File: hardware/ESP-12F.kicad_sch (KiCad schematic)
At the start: 30 parts, among them J10 PROG_PORT, U10 ESP-12F, U11 MCP2558FD-xMF, U8 PI4IOE5V6416LEX, U9 PI4IOE5V6416LEX

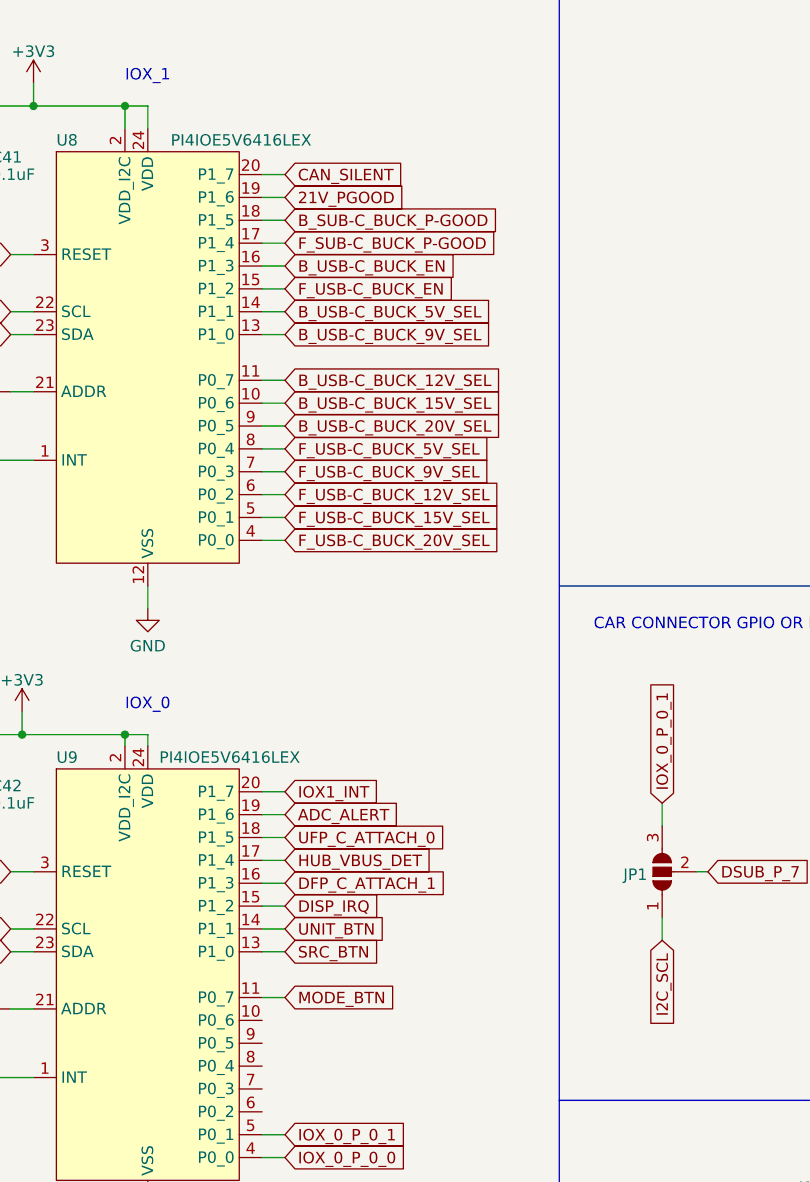
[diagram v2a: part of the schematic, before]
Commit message: coldent sleep so came back and did somre routing
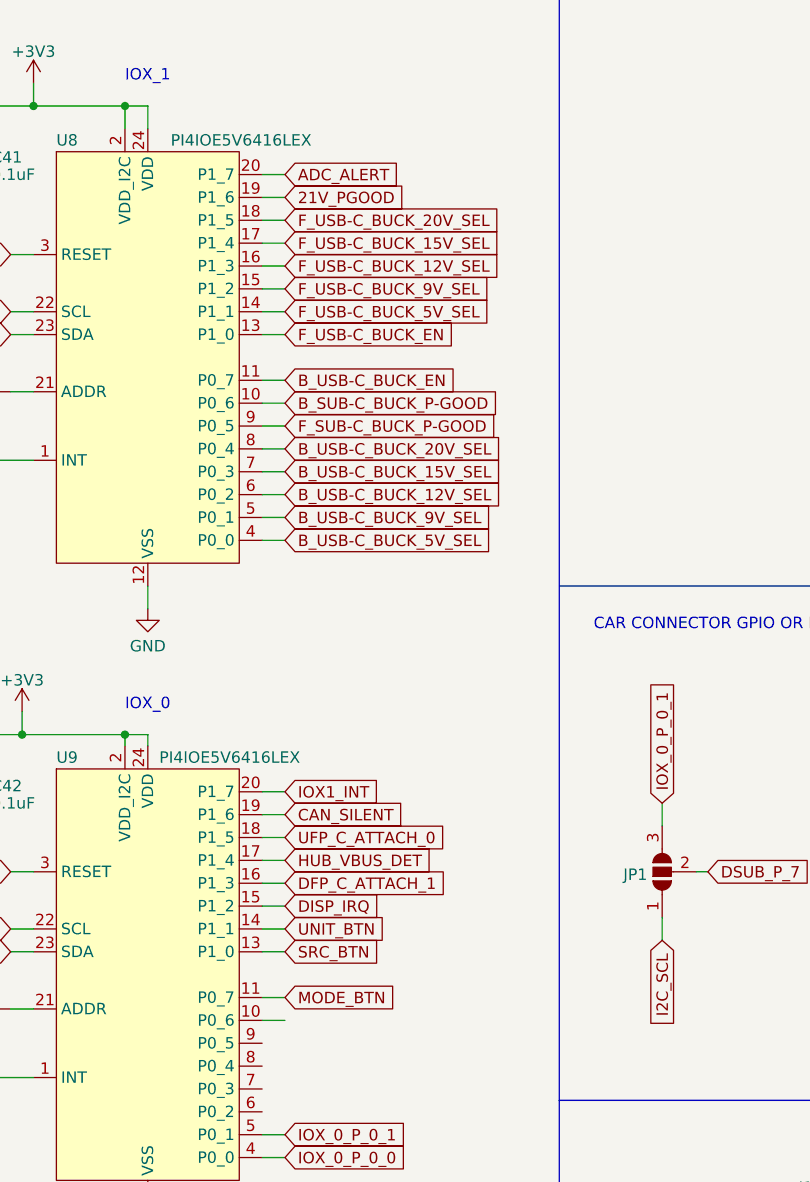
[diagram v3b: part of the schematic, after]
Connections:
- net ADC_ALERT: now also U8.20 (P1_7); no longer U9.19 (P1_6)
- net B_SUB-C_BUCK_P-GOOD: now also U8.10 (P0_6); no longer U8.18 (P1_5)
- net B_USB-C_BUCK_12V_SEL: now also U8.6 (P0_2); no longer U8.11 (P0_7)
- net B_USB-C_BUCK_15V_SEL: now also U8.7 (P0_3); no longer U8.10 (P0_6)
- net B_USB-C_BUCK_20V_SEL: now also U8.8 (P0_4); no longer U8.9 (P0_5)
- net B_USB-C_BUCK_5V_SEL: now also U8.4 (P0_0); no longer U8.14 (P1_1)
- net B_USB-C_BUCK_9V_SEL: now also U8.5 (P0_1); no longer U8.13 (P1_0)
- net B_USB-C_BUCK_EN: now also U8.11 (P0_7); no longer U8.16 (P1_3)
- net CAN_SILENT: now also U9.19 (P1_6); no longer U8.20 (P1_7)
- net F_SUB-C_BUCK_P-GOOD: now also U8.9 (P0_5); no longer U8.17 (P1_4)
- net F_USB-C_BUCK_12V_SEL: now also U8.16 (P1_3); no longer U8.6 (P0_2)
- net F_USB-C_BUCK_15V_SEL: now also U8.17 (P1_4); no longer U8.5 (P0_1)
- net F_USB-C_BUCK_20V_SEL: now also U8.18 (P1_5); no longer U8.4 (P0_0)
- net F_USB-C_BUCK_5V_SEL: now also U8.14 (P1_1); no longer U8.8 (P0_4)
- net F_USB-C_BUCK_9V_SEL: now also U8.15 (P1_2); no longer U8.7 (P0_3)
- net F_USB-C_BUCK_EN: now also U8.13 (P1_0); no longer U8.15 (P1_2)
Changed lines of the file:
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@@
+    (stroke (width 0) (type default))
+  )
+  (wire (pts (xy 82.55 50.8) (xy 85.09 50.8))
     (stroke (width 0) (type default))
   )
@@
     (stroke (width 0) (type default))
   )
+  (wire (pts (xy 82.55 144.78) (xy 85.09 144.78))
+    (stroke (width 0) (type default))
+  )
   (wire (pts (xy 243.84 33.02) (xy 243.84 35.56))
     (stroke (width 0) (type default))
@@
   )
   (wire (pts (xy 38.1 148.59) (xy 38.1 151.13))
-    (stroke (width 0) (type default))
-  )
-  (wire (pts (xy 82.55 50.8) (xy 85.09 50.8))
     (stroke (width 0) (type default))
   )
@@
     )
   )
-  (global_label "B_SUB-C_BUCK_P-GOOD" (shape input) (at 85.09 55.88 0) (fields_autoplaced)
-    (effects (font (size 1.27 1.27)) (justify left))
-    (property "Intersheetrefs" "${INTERSHEET_REFS}" (at 112.0049 55.88 0)
+  (global_label "B_SUB-C_BUCK_P-GOOD" (shape input) (at 85.09 76.2 0) (fields_autoplaced)
+    (effects (font (size 1.27 1.27)) (justify left))
+    (property "Intersheetrefs" "${INTERSHEET_REFS}" (at 112.0049 76.2 0)
       (effects (font (size 1.27 1.27)) (justify left) hide)
     )
@@
     )
   )
-  (global_label "F_USB-C_BUCK_EN" (shape input) (at 85.09 63.5 0) (fields_autoplaced)
-    (effects (font (size 1.27 1.27)) (justify left))
-    (property "Intersheetrefs" "${INTERSHEET_REFS}" (at 106.2596 63.5 0)
-      (effects (font (size 1.27 1.27)) (justify left) hide)
-    )
-  )
-  (global_label "F_USB-C_BUCK_12V_SEL" (shape input) (at 85.09 86.36 0) (fields_autoplaced)
-    (effects (font (size 1.27 1.27)) (justify left))
-    (property "Intersheetrefs" "${INTERSHEET_REFS}" (at 111.6419 86.36 0)
-      (effects (font (size 1.27 1.27)) (justify left) hide)
-    )
-  )
-  (global_label "B_USB-C_BUCK_15V_SEL" (shape input) (at 85.09 76.2 0) (fields_autoplaced)
-    (effects (font (size 1.27 1.27)) (justify left))
-    (property "Intersheetrefs" "${INTERSHEET_REFS}" (at 111.8233 76.2 0)
-      (effects (font (size 1.27 1.27)) (justify left) hide)
-    )
-  )
-  (global_label "F_USB-C_BUCK_5V_SEL" (shape input) (at 85.09 81.28 0) (fields_autoplaced)
-    (effects (font (size 1.27 1.27)) (justify left))
-    (property "Intersheetrefs" "${INTERSHEET_REFS}" (at 110.4324 81.28 0)
+  (global_label "F_USB-C_BUCK_EN" (shape input) (at 85.09 68.58 0) (fields_autoplaced)
+    (effects (font (size 1.27 1.27)) (justify left))
+    (property "Intersheetrefs" "${INTERSHEET_REFS}" (at 106.2596 68.58 0)
+      (effects (font (size 1.27 1.27)) (justify left) hide)
+    )
+  )
+  (global_label "F_USB-C_BUCK_12V_SEL" (shape input) (at 85.09 60.96 0) (fields_autoplaced)
+    (effects (font (size 1.27 1.27)) (justify left))
+    (property "Intersheetrefs" "${INTERSHEET_REFS}" (at 111.6419 60.96 0)
+      (effects (font (size 1.27 1.27)) (justify left) hide)
+    )
+  )
+  (global_label "B_USB-C_BUCK_15V_SEL" (shape input) (at 85.09 83.82 0) (fields_autoplaced)
+    (effects (font (size 1.27 1.27)) (justify left))
+    (property "Intersheetrefs" "${INTERSHEET_REFS}" (at 111.8233 83.82 0)
+      (effects (font (size 1.27 1.27)) (justify left) hide)
+    )
+  )
+  (global_label "F_USB-C_BUCK_5V_SEL" (shape input) (at 85.09 66.04 0) (fields_autoplaced)
+    (effects (font (size 1.27 1.27)) (justify left))
+    (property "Intersheetrefs" "${INTERSHEET_REFS}" (at 110.4324 66.04 0)
       (effects (font (size 1.27 1.27)) (justify left) hide)
     )
@@
     )
   )
-  (global_label "B_USB-C_BUCK_5V_SEL" (shape input) (at 85.09 66.04 0) (fields_autoplaced)
-    (effects (font (size 1.27 1.27)) (justify left))
-    (property "Intersheetrefs" "${INTERSHEET_REFS}" (at 110.6138 66.04 0)
+  (global_label "B_USB-C_BUCK_5V_SEL" (shape input) (at 85.09 91.44 0) (fields_autoplaced)
+    (effects (font (size 1.27 1.27)) (justify left))
+    (property "Intersheetrefs" "${INTERSHEET_REFS}" (at 110.6138 91.44 0)
       (effects (font (size 1.27 1.27)) (justify left) hide)
     )
@@
     )
   )
-  (global_label "F_USB-C_BUCK_9V_SEL" (shape input) (at 85.09 83.82 0) (fields_autoplaced)
-    (effects (font (size 1.27 1.27)) (justify left))
-    (property "Intersheetrefs" "${INTERSHEET_REFS}" (at 110.4324 83.82 0)
+  (global_label "F_USB-C_BUCK_9V_SEL" (shape input) (at 85.09 63.5 0) (fields_autoplaced)
+    (effects (font (size 1.27 1.27)) (justify left))
+    (property "Intersheetrefs" "${INTERSHEET_REFS}" (at 110.4324 63.5 0)
       (effects (font (size 1.27 1.27)) (justify left) hide)
     )
@@
     )
   )
-  (global_label "B_USB-C_BUCK_20V_SEL" (shape input) (at 85.09 78.74 0) (fields_autoplaced)
-    (effects (font (size 1.27 1.27)) (justify left))
-    (property "Intersheetrefs" "${INTERSHEET_REFS}" (at 111.8233 78.74 0)
+  (global_label "B_USB-C_BUCK_20V_SEL" (shape input) (at 85.09 81.28 0) (fields_autoplaced)
+    (effects (font (size 1.27 1.27)) (justify left))
+    (property "Intersheetrefs" "${INTERSHEET_REFS}" (at 111.8233 81.28 0)
       (effects (font (size 1.27 1.27)) (justify left) hide)
     )
@@
     )
   )
-  (global_label "ADC_ALERT" (shape input) (at 85.09 121.92 0) (fields_autoplaced)
-    (effects (font (size 1.27 1.27)) (justify left))
-    (property "Intersheetrefs" "${INTERSHEET_REFS}" (at 98.0953 121.92 0)
-      (effects (font (size 1.27 1.27)) (justify left) hide)
-    )
-  )
-  (global_label "F_USB-C_BUCK_15V_SEL" (shape input) (at 85.09 88.9 0) (fields_autoplaced)
-    (effects (font (size 1.27 1.27)) (justify left))
-    (property "Intersheetrefs" "${INTERSHEET_REFS}" (at 111.6419 88.9 0)
+  (global_label "ADC_ALERT" (shape input) (at 85.09 50.8 0) (fields_autoplaced)
+    (effects (font (size 1.27 1.27)) (justify left))
+    (property "Intersheetrefs" "${INTERSHEET_REFS}" (at 98.0953 50.8 0)
+      (effects (font (size 1.27 1.27)) (justify left) hide)
+    )
+  )
+  (global_label "F_USB-C_BUCK_15V_SEL" (shape input) (at 85.09 58.42 0) (fields_autoplaced)
+    (effects (font (size 1.27 1.27)) (justify left))
+    (property "Intersheetrefs" "${INTERSHEET_REFS}" (at 111.6419 58.42 0)
       (effects (font (size 1.27 1.27)) (justify left) hide)
     )
@@
     )
   )
-  (global_label "B_USB-C_BUCK_9V_SEL" (shape input) (at 85.09 68.58 0) (fields_autoplaced)
-    (effects (font (size 1.27 1.27)) (justify left))
-    (property "Intersheetrefs" "${INTERSHEET_REFS}" (at 110.6138 68.58 0)
+  (global_label "B_USB-C_BUCK_9V_SEL" (shape input) (at 85.09 88.9 0) (fields_autoplaced)
+    (effects (font (size 1.27 1.27)) (justify left))
+    (property "Intersheetrefs" "${INTERSHEET_REFS}" (at 110.6138 88.9 0)
       (effects (font (size 1.27 1.27)) (justify left) hide)
     )
@@
     )
   )
-  (global_label "B_USB-C_BUCK_12V_SEL" (shape input) (at 85.09 73.66 0) (fields_autoplaced)
-    (effects (font (size 1.27 1.27)) (justify left))
-    (property "Intersheetrefs" "${INTERSHEET_REFS}" (at 111.8233 73.66 0)
+  (global_label "B_USB-C_BUCK_12V_SEL" (shape input) (at 85.09 86.36 0) (fields_autoplaced)
+    (effects (font (size 1.27 1.27)) (justify left))
+    (property "Intersheetrefs" "${INTERSHEET_REFS}" (at 111.8233 86.36 0)
       (effects (font (size 1.27 1.27)) (justify left) hide)
     )
@@
     )
   )
-  (global_label "CAN_SILENT" (shape input) (at 85.09 50.8 0) (fields_autoplaced)
-    (effects (font (size 1.27 1.27)) (justify left))
-    (property "Intersheetrefs" "${INTERSHEET_REFS}" (at 98.942 50.8 0)
+  (global_label "CAN_SILENT" (shape input) (at 85.09 121.92 0) (fields_autoplaced)
+    (effects (font (size 1.27 1.27)) (justify left))
+    (property "Intersheetrefs" "${INTERSHEET_REFS}" (at 98.942 121.92 0)
       (effects (font (size 1.27 1.27)) (justify left) hide)
     )
@@
     )
   )
-  (global_label "F_SUB-C_BUCK_P-GOOD" (shape input) (at 85.09 58.42 0) (fields_autoplaced)
-    (effects (font (size 1.27 1.27)) (justify left))
-    (property "Intersheetrefs" "${INTERSHEET_REFS}" (at 111.8235 58.42 0)
+  (global_label "F_SUB-C_BUCK_P-GOOD" (shape input) (at 85.09 78.74 0) (fields_autoplaced)
+    (effects (font (size 1.27 1.27)) (justify left))
+    (property "Intersheetrefs" "${INTERSHEET_REFS}" (at 111.8235 78.74 0)
       (effects (font (size 1.27 1.27)) (justify left) hide)
     )
@@
     )
   )
-  (global_label "B_USB-C_BUCK_EN" (shape input) (at 85.09 60.96 0) (fields_autoplaced)
-    (effects (font (size 1.27 1.27)) (justify left))
-    (property "Intersheetrefs" "${INTERSHEET_REFS}" (at 106.441 60.96 0)
+  (global_label "B_USB-C_BUCK_EN" (shape input) (at 85.09 73.66 0) (fields_autoplaced)
+    (effects (font (size 1.27 1.27)) (justify left))
+    (property "Intersheetrefs" "${INTERSHEET_REFS}" (at 106.441 73.66 0)
       (effects (font (size 1.27 1.27)) (justify left) hide)
     )
@@
     )
   )
-  (global_label "F_USB-C_BUCK_20V_SEL" (shape input) (at 85.09 91.44 0) (fields_autoplaced)
-    (effects (font (size 1.27 1.27)) (justify left))
-    (property "Intersheetrefs" "${INTERSHEET_REFS}" (at 111.6419 91.44 0)
-      (effects (font (size 1.27 1.27)) (justify left) hide)
-    )
+  (global_label "F_USB-C_BUCK_20V_SEL" (shape input) (at 85.09 55.88 0) (fields_autoplaced)
+    (effects (font (size 1.27 1.27)) (justify left))
+    (property "Intersheetrefs" "${INTERSHEET_REFS}" (at 111.6419 55.88 0)
+      (effects (font (size 1.27 1.27)) (justify left) hide)
+    )
